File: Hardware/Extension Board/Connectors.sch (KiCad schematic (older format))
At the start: 25 parts, among them J11 TUNE, J12 BUS I2C, J15 CNX LEDS, J16 BUS I2C, J4 BUS SPI, J5 MODE, J7 I/O SPARE, J8 NEXT_AGAIN, U3 74HC14

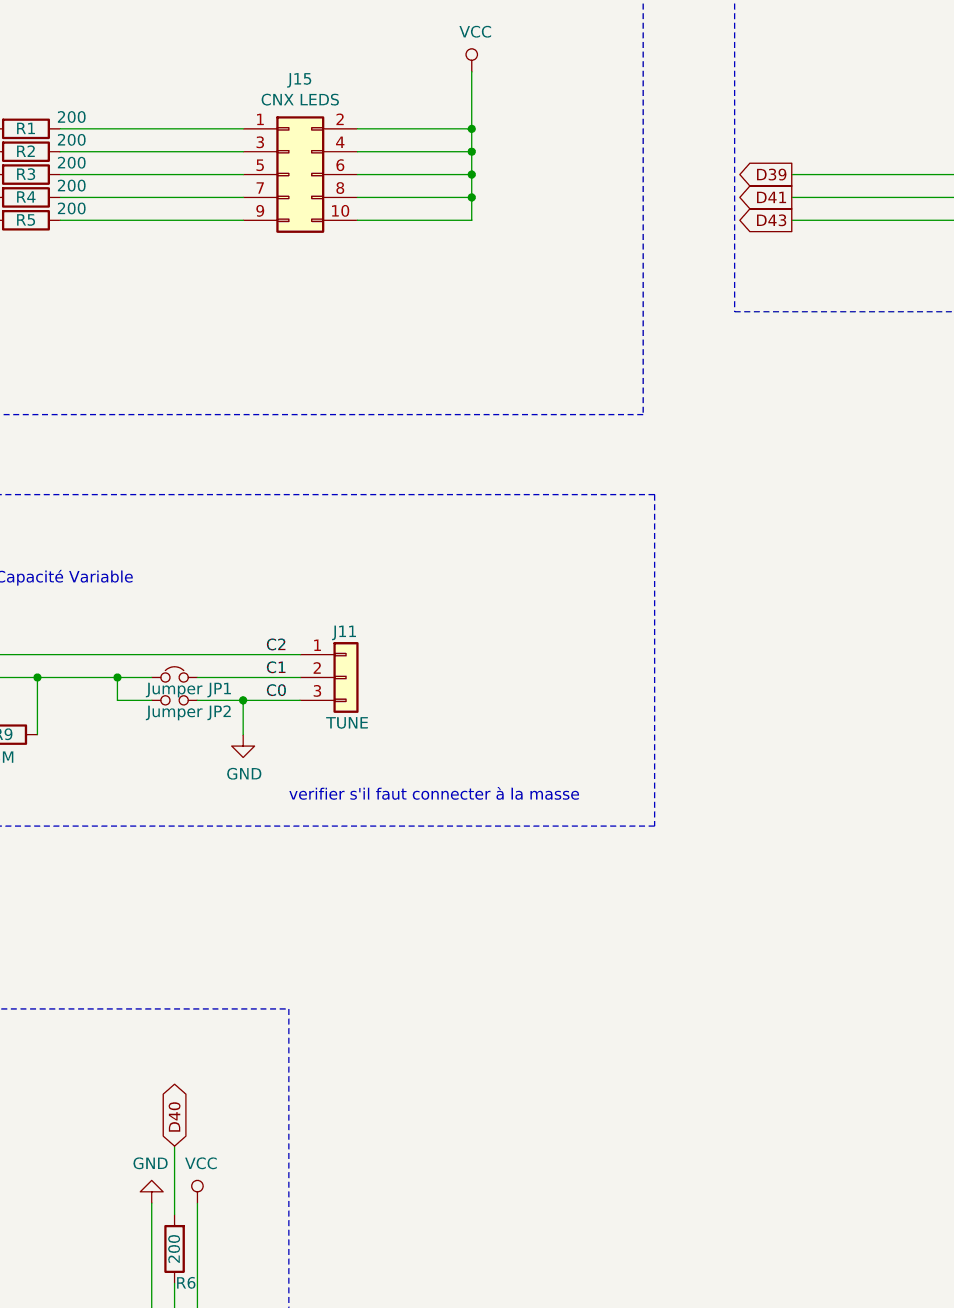
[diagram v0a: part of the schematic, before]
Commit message: Routage du PCB
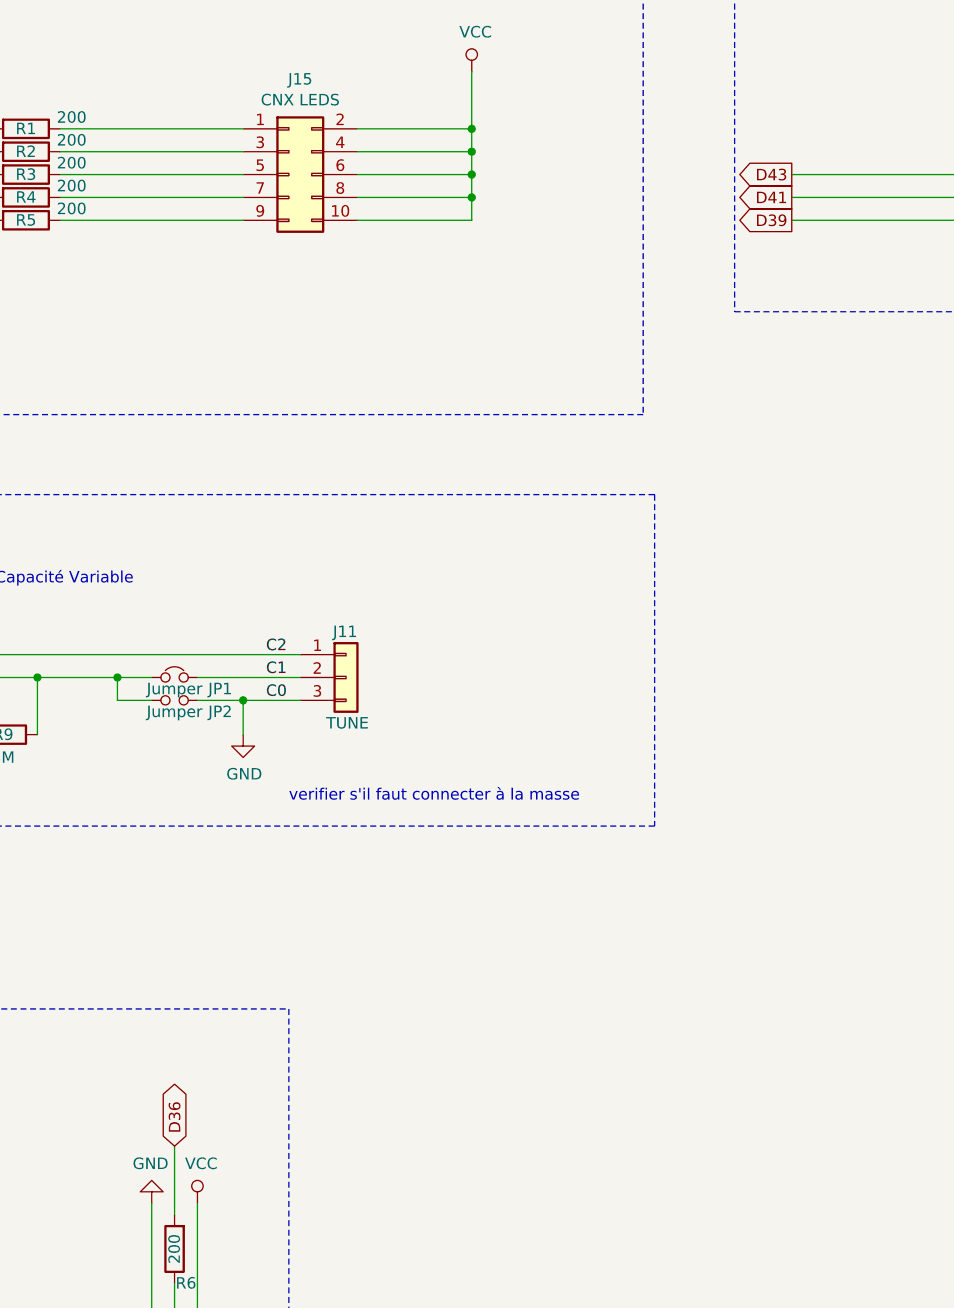
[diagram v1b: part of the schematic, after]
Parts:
- R9: footprint Resistor_THT:R_Axial_DIN0414_L11.9mm_D4.5mm_P20.32mm_Horizontal -> Resistor_THT:R_Axial_DIN0309_L9.0mm_D3.2mm_P15.24mm_Horizontal
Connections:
- net D39: now also J5.2 (Pin_2), RN1.4 (R3); no longer J5.4 (Pin_4), RN1.2 (R1)
- net D43: now also J5.4 (Pin_4), RN1.2 (R1); no longer J5.2 (Pin_2), RN1.4 (R3)
- net D40 renamed D36
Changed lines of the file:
@@
 	2800 6250 2800 5950
 Text GLabel 2800 5950 1    50   BiDi ~ 0
-D40
+D36
 Text Notes 1100 5500 0    50   ~ 0
 Spare connectors
@@
 $EndComp
 Text GLabel 5500 1900 0    50   Output ~ 0
-D43
+D39
 Text GLabel 5500 1800 0    50   Output ~ 0
 D41
 Text GLabel 5500 1700 0    50   Output ~ 0
-D39
+D43
 Connection ~ 6400 1700
 Wire Wire Line
@@
 F 0 "R9" V 2050 4150 50  0000 C CNN
 F 1 "3M" V 2150 4150 50  0000 C CNN
-F 2 "Resistor_THT:R_Axial_DIN0414_L11.9mm_D4.5mm_P20.32mm_Horizontal" V 1980 4150 50  0001 C CNN
+F 2 "Resistor_THT:R_Axial_DIN0309_L9.0mm_D3.2mm_P15.24mm_Horizontal" V 1980 4150 50  0001 C CNN
 F 3 "~" H 2050 4150 50  0001 C CNN
 	1    2050 4150
